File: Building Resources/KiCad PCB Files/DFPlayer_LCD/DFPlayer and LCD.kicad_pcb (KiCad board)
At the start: 2 copper layers, 30.3 x 21.7 mm, 2 parts, among them J1 Conn_01x06_Socket, U1 DFR0299

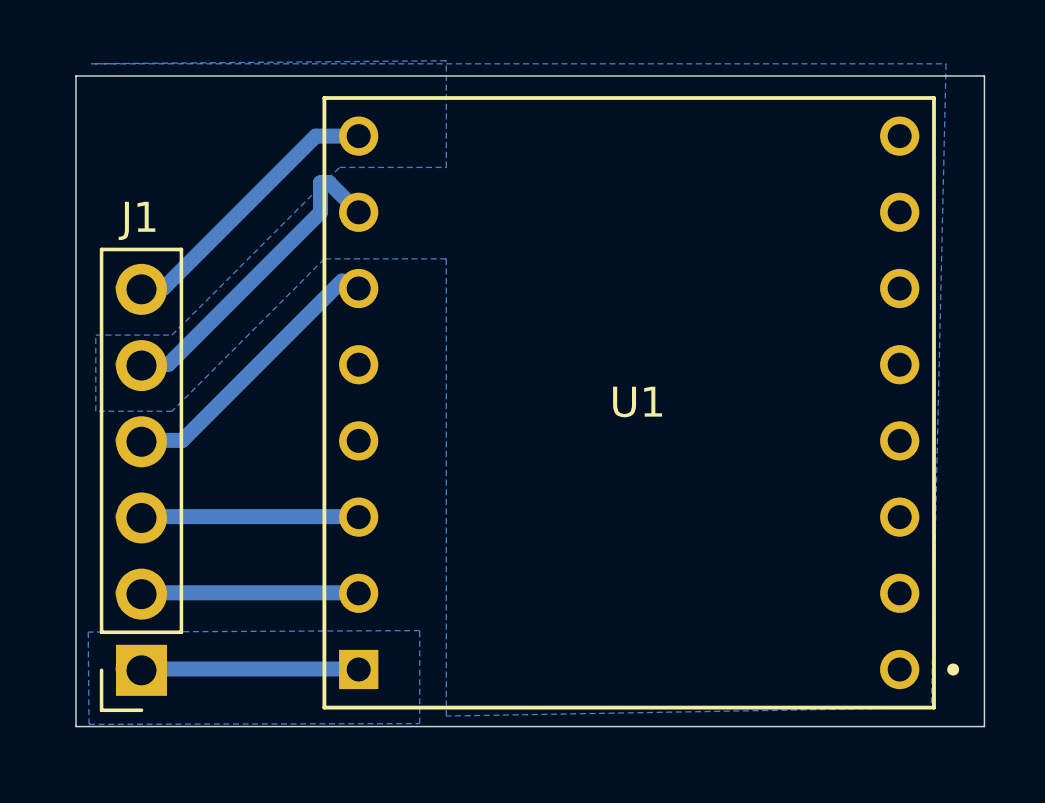
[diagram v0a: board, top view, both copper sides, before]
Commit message: More updates, finally.
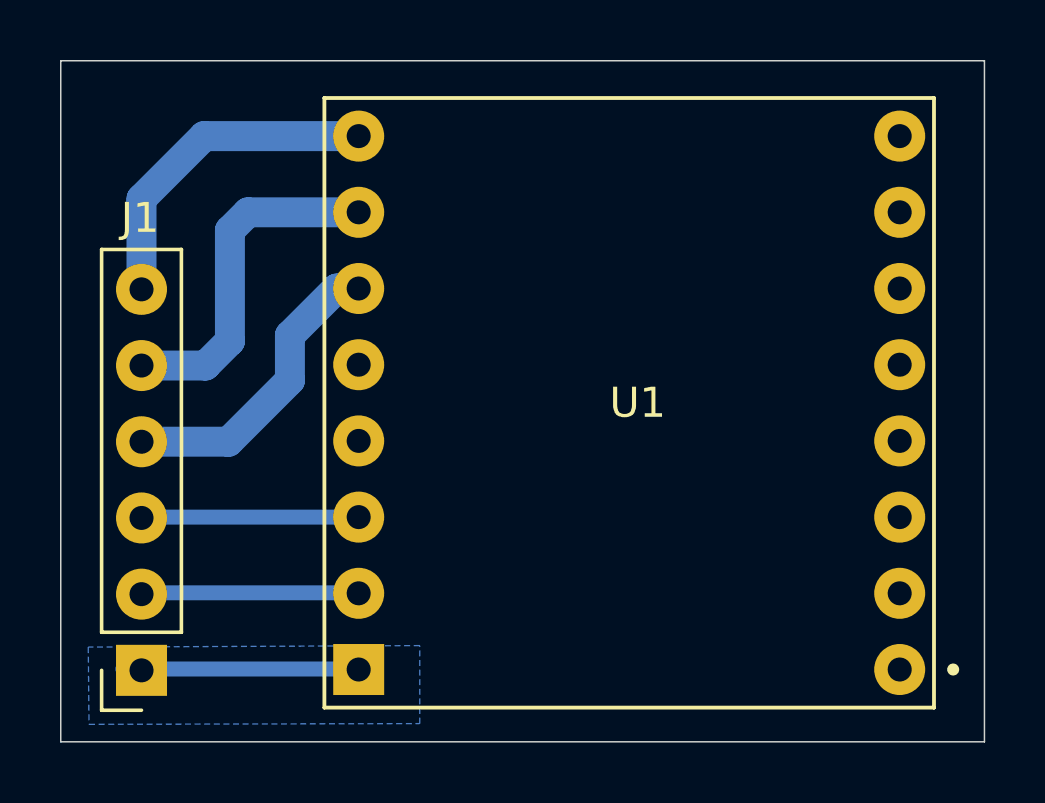
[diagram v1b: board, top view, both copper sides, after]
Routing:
- net Net-(J1-Pin_6): track 9.96 -> 11.1 mm
- net Net-(J1-Pin_4): track 9.51 -> 10.2 mm
- net Net-(J1-Pin_3): track 7.34 -> 6.71 mm
- removed copper zone on B.Cu, net Net-(J1-Pin_5)
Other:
- board size 30.3 x 21.7 mm -> 30.8 x 22.7 mm
